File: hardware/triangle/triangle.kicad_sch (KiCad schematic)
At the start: 55 parts, among them J1 Conn_01x02_Socket, J2 Conn_01x02_Socket

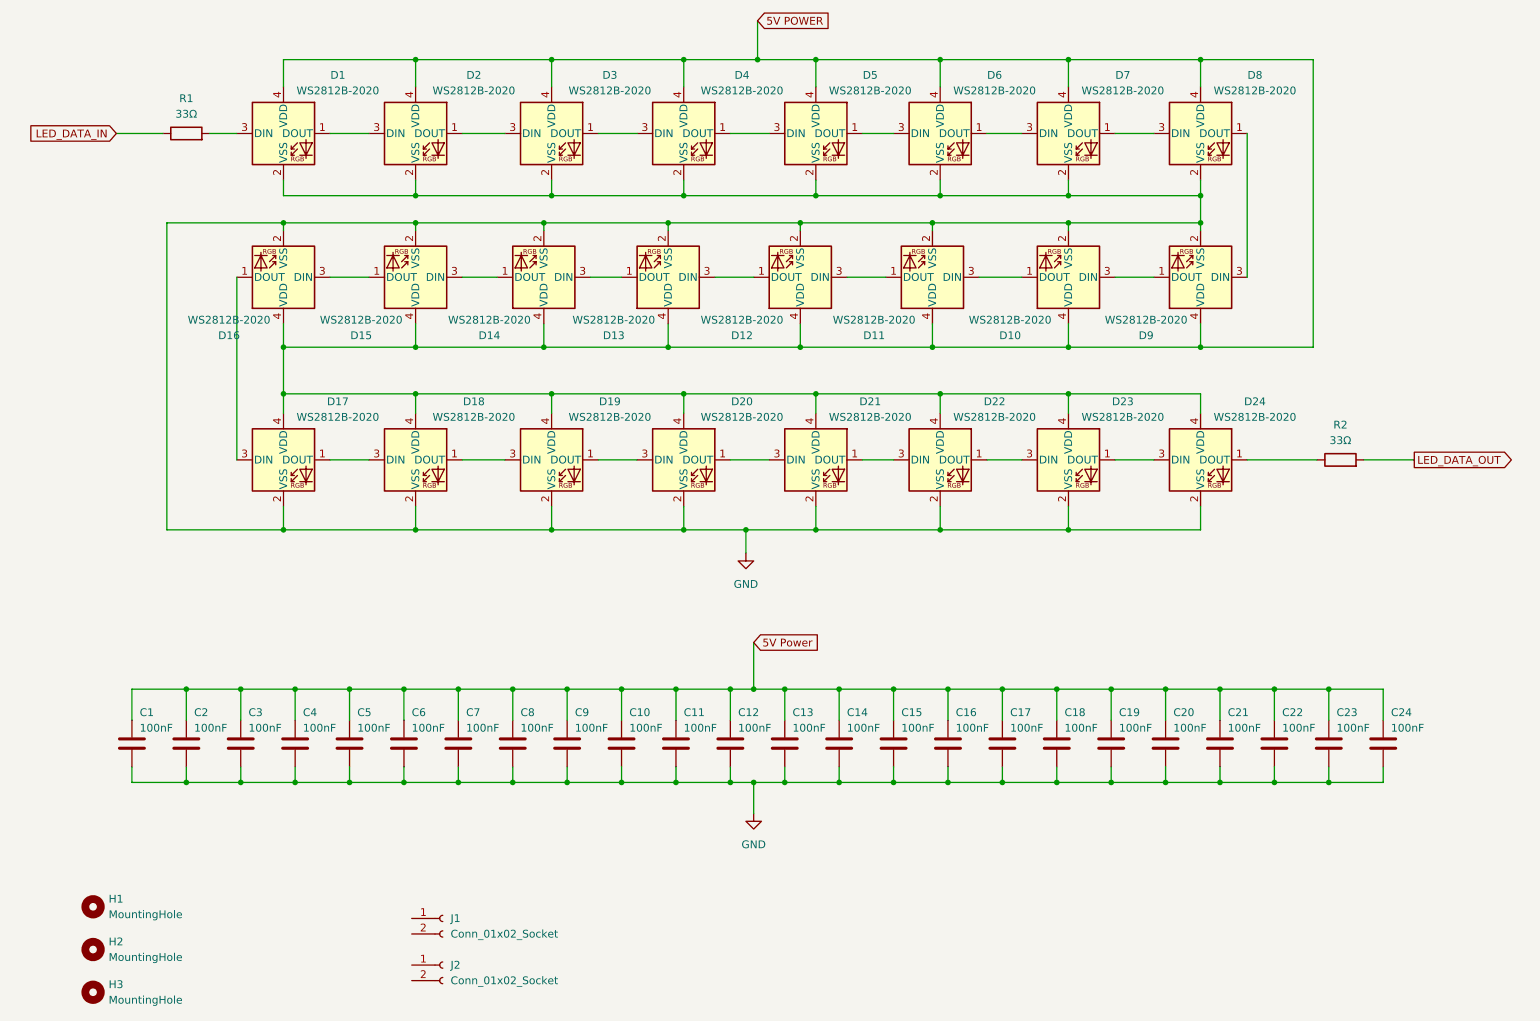
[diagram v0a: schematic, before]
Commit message: routing efforts for the triangle
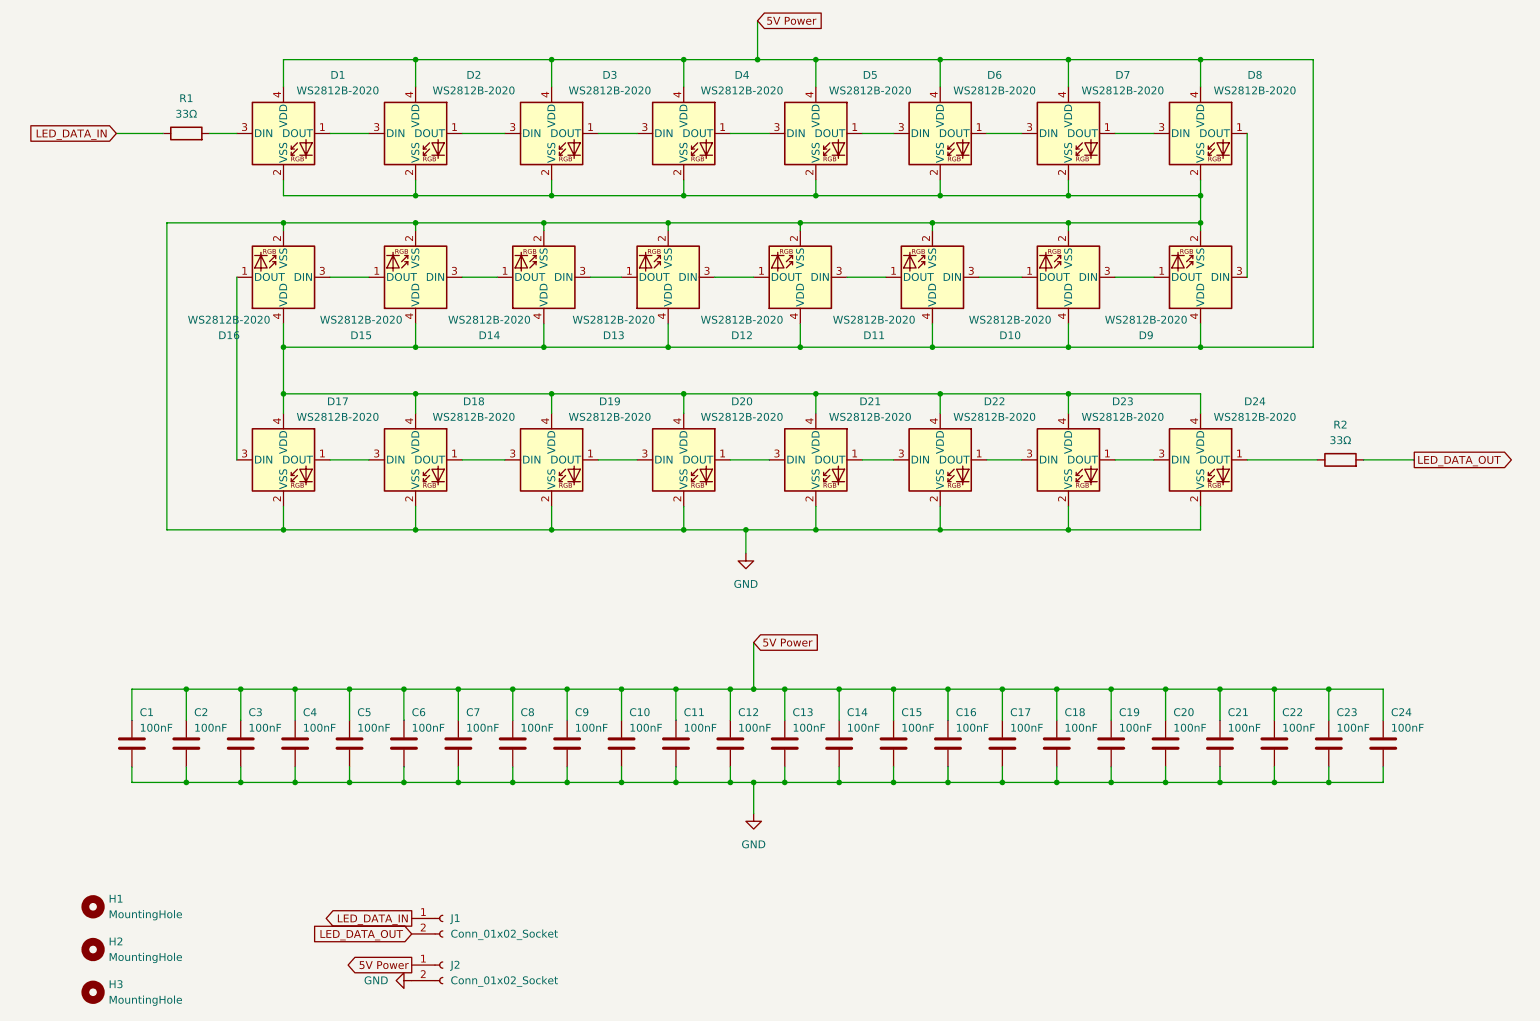
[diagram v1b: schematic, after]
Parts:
- J1, J2: footprint Connector_JST:JST_PH_S2B-PH-SM4-TB_1x02-1MP_P2.00mm_Horizontal -> footprints:CONN-SMD_ZX-XH2.54-2PLT; JLCPCB Part # (none) -> C7429680
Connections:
- net 5V POWER is gone; now on net 5V Power: D1.4 (VDD), D10.4 (VDD), D11.4 (VDD), D12.4 (VDD), D13.4 (VDD), D14.4 (VDD), D15.4 (VDD), D16.4 (VDD), D17.4 (VDD), D18.4 (VDD), D19.4 (VDD), D2.4 (VDD), D20.4 (VDD), D21.4 (VDD), D22.4 (VDD), D23.4 (VDD), D24.4 (VDD), D3.4 (VDD), D4.4 (VDD), D5.4 (VDD), D6.4 (VDD), D7.4 (VDD), D8.4 (VDD), D9.4 (VDD)
- net 5V Power: now also J2.1 (Pin_1)
- net GND: now also J2.2 (Pin_2)
- net LED_DATA_IN: now also J1.1 (Pin_1)
- net LED_DATA_OUT: now also J1.2 (Pin_2)
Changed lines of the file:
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@@
 		)
 	)
-	(global_label "5V POWER"
+	(global_label "5V Power"
+		(shape output)
+		(at 93.98 173.355 180)
+		(fields_autoplaced yes)
+		(effects
+			(font
+				(size 1.27 1.27)
+			)
+			(justify right)
+		)
+		(property "Intersheetrefs" "${INTERSHEET_REFS}"
+			(at 82.1048 173.355 0)
+			(hide yes)
+			(show_name no)
+			(do_not_autoplace no)
+			(effects
+				(font
+					(size 1.27 1.27)
+				)
+				(justify right)
+			)
+		)
+	)
+	(global_label "5V Power"
 		(shape input)
 		(at 150.495 19.05 0)
@@
 		)
 		(property "Intersheetrefs" "${INTERSHEET_REFS}"
-			(at 163.2168 19.05 0)
+			(at 162.3702 19.05 0)
 			(hide yes)
 			(show_name no)
@@
 		)
 	)
+	(global_label "LED_DATA_OUT"
+		(shape input)
+		(at 93.98 168.275 180)
+		(fields_autoplaced yes)
+		(effects
+			(font
+				(size 1.27 1.27)
+			)
+			(justify right)
+		)
+		(property "Intersheetrefs" "${INTERSHEET_REFS}"
+			(at 77.5691 168.275 0)
+			(hide yes)
+			(show_name no)
+			(do_not_autoplace no)
+			(effects
+				(font
+					(size 1.27 1.27)
+				)
+				(justify right)
+			)
+		)
+	)
+	(global_label "LED_DATA_IN"
+		(shape output)
+		(at 93.98 165.735 180)
+		(fields_autoplaced yes)
+		(effects
+			(font
+				(size 1.27 1.27)
+			)
+			(justify right)
+		)
+		(property "Intersheetrefs" "${INTERSHEET_REFS}"
+			(at 79.2624 165.735 0)
+			(hide yes)
+			(show_name no)
+			(do_not_autoplace no)
+			(effects
+				(font
+					(size 1.27 1.27)
+				)
+				(justify right)
+			)
+		)
+	)
 	(global_label "LED_DATA_IN"
 		(shape input)
@@
 			)
 		)
-		(property "Footprint" "Connector_JST:JST_PH_S2B-PH-SM4-TB_1x02-1MP_P2.00mm_Horizontal"
+		(property "Footprint" "footprints:CONN-SMD_ZX-XH2.54-2PLT"
 			(at 99.06 173.355 0)
 			(hide yes)
@@
 			)
 		)
+		(property "JLCPCB Part #" "C7429680"
+			(at 99.06 173.355 0)
+			(hide yes)
+			(show_name no)
+			(do_not_autoplace no)
+			(effects
+				(font
+					(size 1.27 1.27)
+				)
+			)
+		)
 		(pin "2"
 		)
@@
 			)
 		)
-		(property "Footprint" "Connector_JST:JST_PH_S2B-PH-SM4-TB_1x02-1MP_P2.00mm_Horizontal"
+		(property "Footprint" "footprints:CONN-SMD_ZX-XH2.54-2PLT"
 			(at 99.06 165.735 0)
 			(hide yes)
@@
 			)
 		)
+		(property "JLCPCB Part #" "C7429680"
+			(at 99.06 165.735 0)
+			(hide yes)
+			(show_name no)
+			(do_not_autoplace no)
+			(effects
+				(font
+					(size 1.27 1.27)
+				)
+			)
+		)
 		(pin "2"
 		)
@@
 					(unit 1)
 				)
+			)
+		)
+	)
+	(symbol
+		(lib_id "power:GND")
+		(at 93.98 175.895 270)
+		(unit 1)
+		(body_style 1)
+		(exclude_from_sim no)
+		(in_bom yes)
+		(on_board yes)
+		(in_pos_files yes)
+		(dnp no)
+		(fields_autoplaced yes)
+		(property "Reference" "#PWR01"
+			(at 87.63 175.895 0)
+			(hide yes)
+			(show_name no)
+			(do_not_autoplace no)
+			(effects
+				(font
+					(size 1.27 1.27)
+				)
+			)
+		)
+		(property "Value" "GND"
+			(at 90.17 175.8949 90)
+			(show_name no)
+			(do_not_autoplace no)
+			(effects
+				(font
+					(size 1.27 1.27)
+				)
+				(justify right)
+			)
+		)
+		(property "Footprint" ""
+			(at 93.98 175.895 0)
+			(hide yes)
+			(show_name no)
+			(do_not_autoplace no)
+			(effects
+				(font
+					(size 1.27 1.27)
+				)
+			)
+		)
+		(property "Datasheet" ""
+			(at 93.98 175.895 0)
+			(hide yes)
+			(show_name no)
+			(do_not_autoplace no)
+			(effects
+				(font
+					(size 1.27 1.27)
+				)
+			)
+		)
+		(property "Description" "Power symbol creates a global label with name \"GND\" , ground"
+			(at 93.98 175.895 0)
+			(hide yes)
+			(show_name no)
+			(do_not_autoplace no)
+			(effects
+				(font
+					(size 1.27 1.27)
+				)
+			)
+		)
+		(pin "1"
+		)
+		(instances
+			(project "triangle"
+				(path "/f9839f04-8b32-4f6f-9cb5-92c3ed04dc78"
+					(reference "#PWR01")
+					(unit 1)
+				)
